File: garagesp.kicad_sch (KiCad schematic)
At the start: 20 parts, among them J1 USB_C_Receptacle_USB2.0_14P, J2 AHT21, J3 DOOR CTL, J4 DOOR SW, K1 SANYOU_SRD_Form_C, Q1 BC547, SW1 RESET, SW2 BOOT, U1 ESP32-C3-WROOM-02, U2 AP2112K-3.3

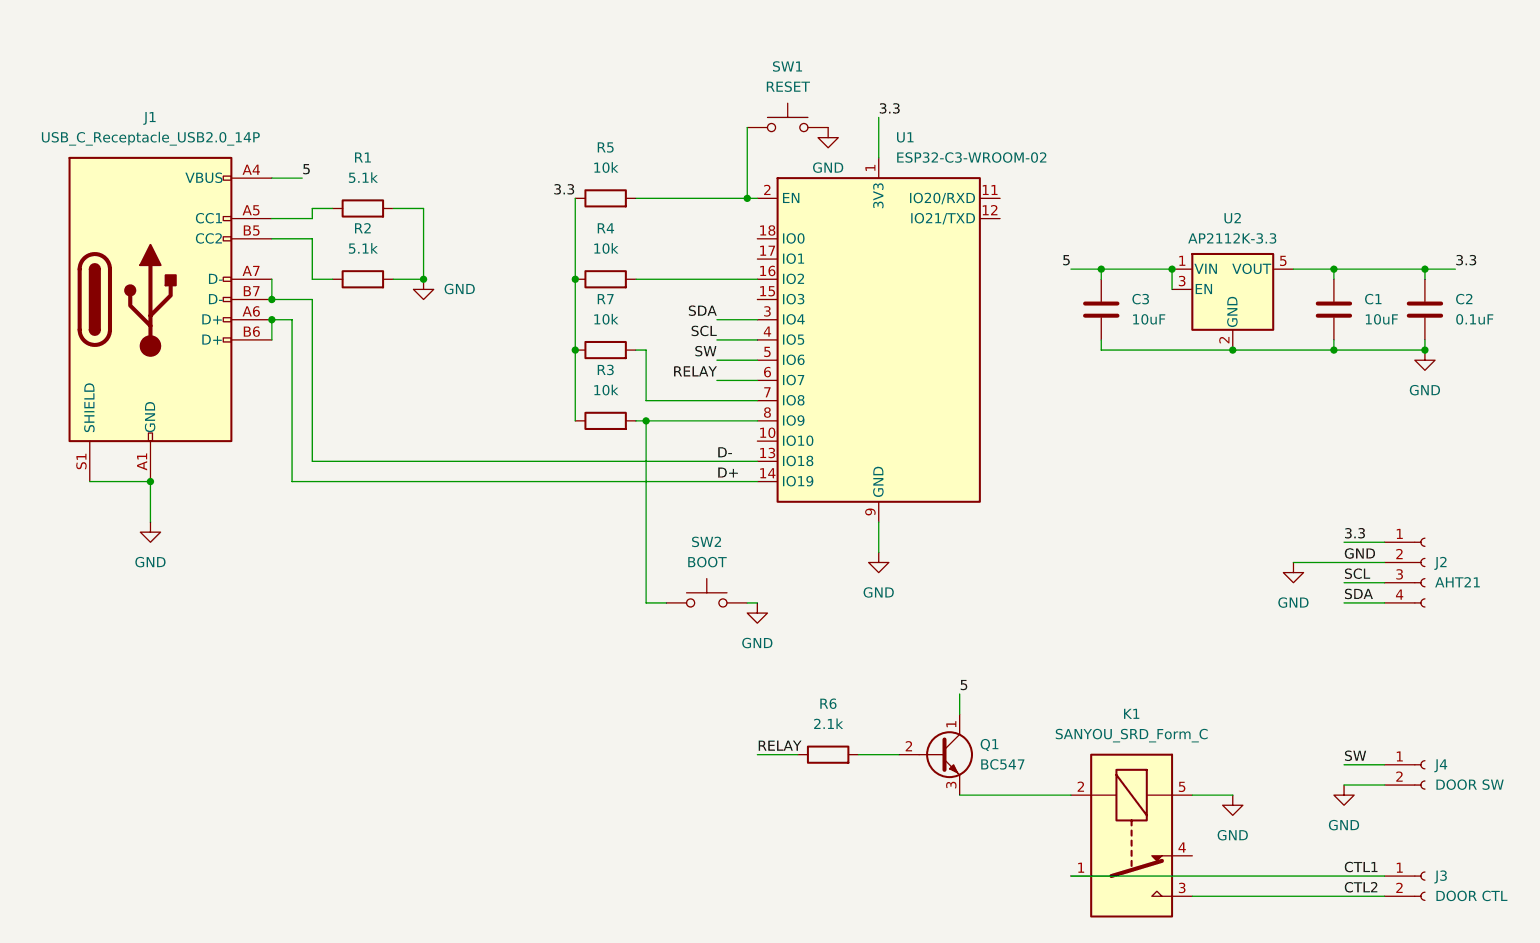
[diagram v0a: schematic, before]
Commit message: move things around again
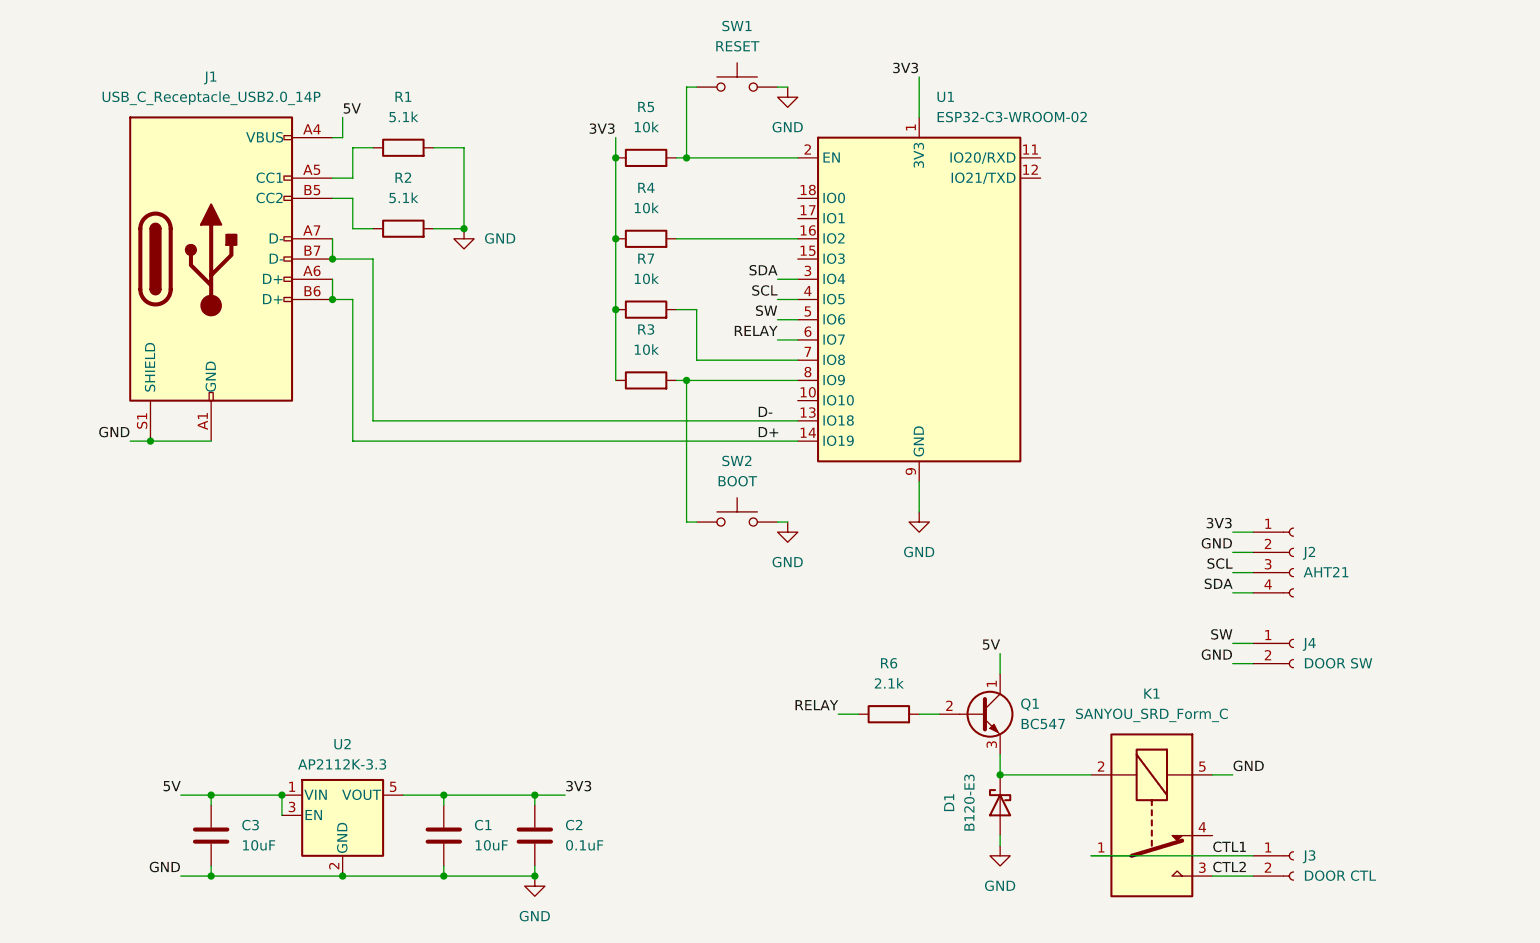
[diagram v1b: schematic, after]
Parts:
- added D1: B120-E3, Diode_SMD:D_SMA, symbol Diode:B120-E3
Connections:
- net GND: now also D1.2 (A)
- net at K1.2, Q1.3 (E): now also D1.1 (K)
- net 3.3 renamed 3V3
- net 5 renamed 5V
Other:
- moved on the sheet: C1, C2, C3, J1, J2, J3, J4, K1, Q1, R1, R2, R3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
